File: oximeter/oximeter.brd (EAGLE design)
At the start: 29 x 41 mm, 24 parts, among them U1 AFE4490_AFE4490, U2 AZ1117EH-3.3TRG1, X1 FFC-32

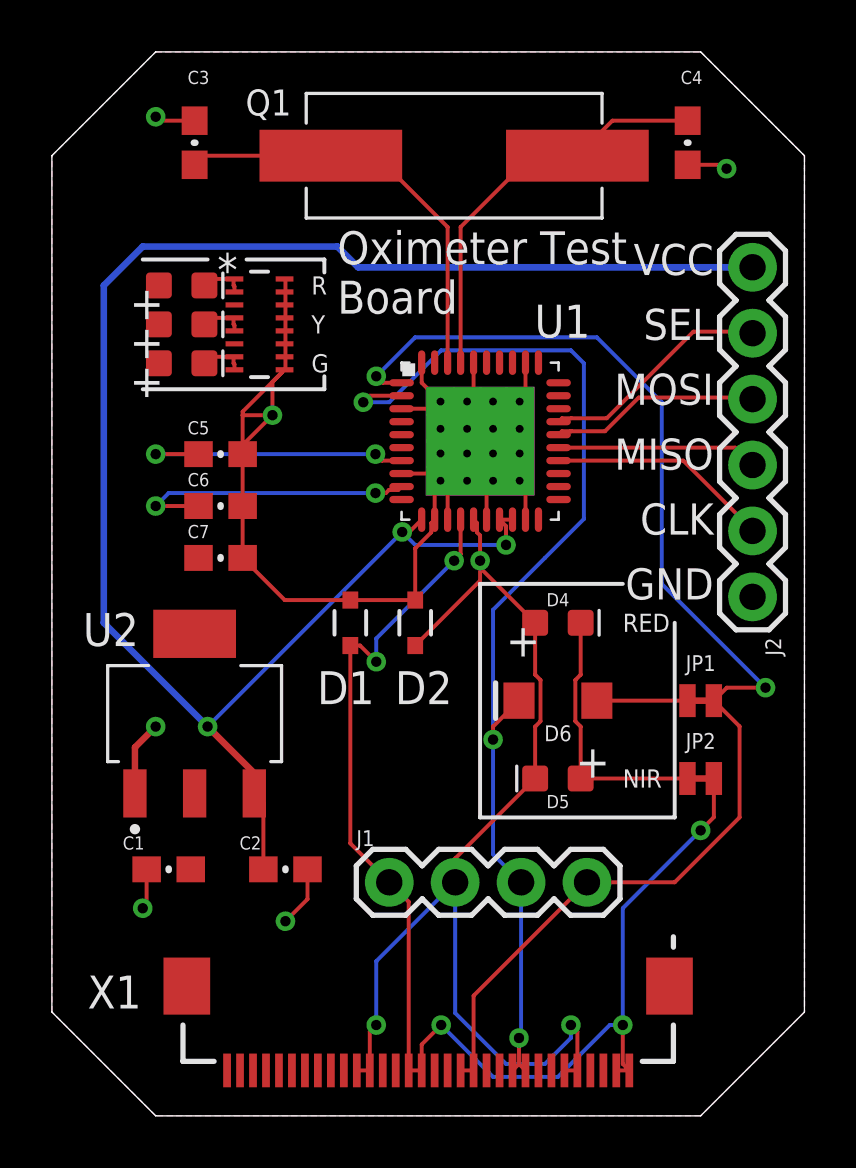
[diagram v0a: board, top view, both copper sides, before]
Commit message: more nextflex progress
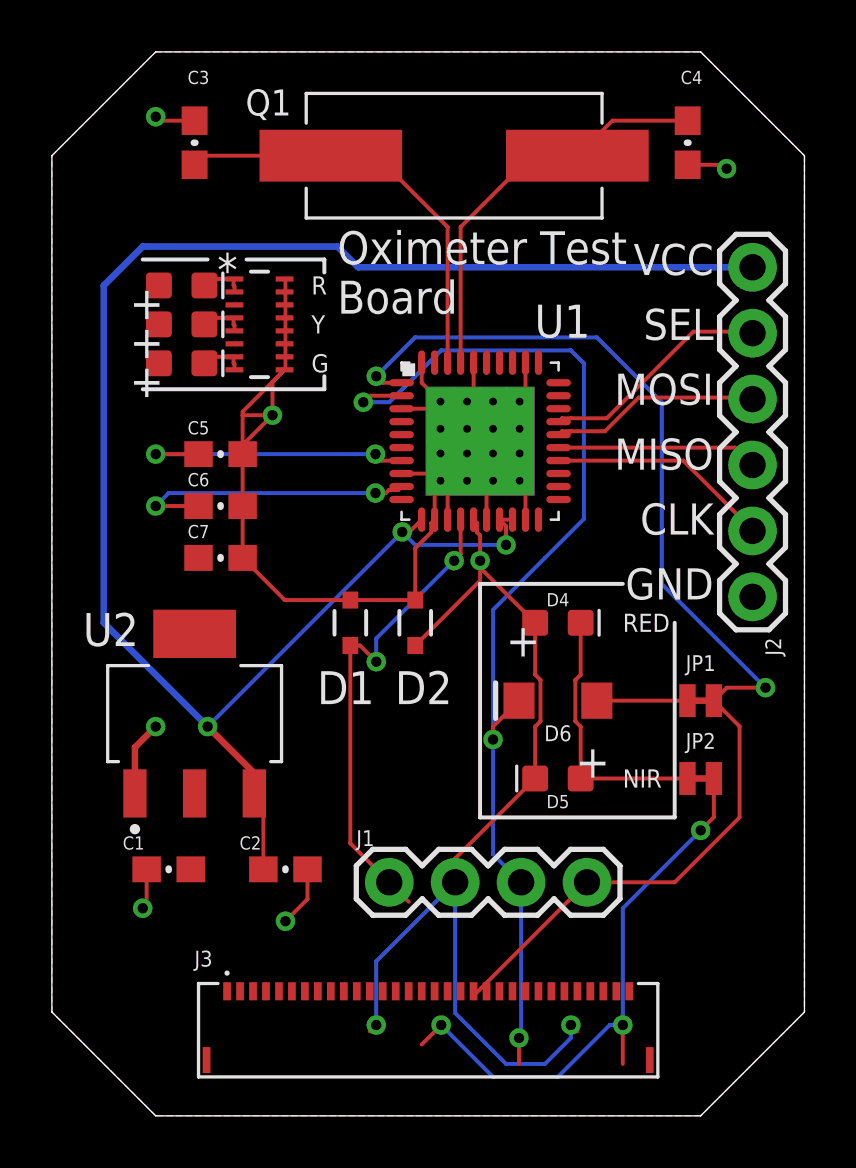
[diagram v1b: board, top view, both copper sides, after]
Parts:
- removed X1: FFC-32, scono:5034803200
- added J3: FFC-32, scono:MOLEX_503480-3200
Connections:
- new net N$1: J3.31
- new net N$2: J3.15
- new net N$3: J3.27
- new net N$4: J3.11
- new net N$8: J3.19
- new net N$9: J3.23
- net INN: now also J3.20; no longer X1.13, X1.14
- net INP: now also J3.24; no longer X1.10, X1.9
- net TXN: now also J3.16, J3.32; no longer X1.1, X1.17, X1.18, X1.2
- net TXP: now also J3.12, J3.28; no longer X1.21, X1.22, X1.5, X1.6
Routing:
- net TXN: track 49.9 -> 41.1 mm
- net TXP: track 43.4 -> 39.4 mm
- net INN: track 50.0 -> 46.6 mm
- net INP: track 42.7 -> 42.0 mm
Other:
- outline, holes or cut-outs redrawn
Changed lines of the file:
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@@
 <?xml version="1.0" encoding="utf-8"?>
 <!DOCTYPE eagle SYSTEM "eagle.dtd">
-<eagle version="9.4.2">
+<eagle version="9.5.1">
 <drawing>
 <settings>
@@
 <layer number="154" name="FabDoc2" color="7" fill="1" visible="yes" active="yes"/>
 <layer number="155" name="FabDoc3" color="7" fill="1" visible="yes" active="yes"/>
+<layer number="166" name="AntennaArea" color="7" fill="1" visible="no" active="yes"/>
+<layer number="168" name="4mmHeightArea" color="7" fill="1" visible="no" active="yes"/>
 <layer number="191" name="mNets" color="7" fill="1" visible="yes" active="yes"/>
 <layer number="192" name="mBusses" color="7" fill="1" visible="yes" active="yes"/>
@@
 <wire x1="3" y1="0" x2="24" y2="0" width="0" layer="20"/>
 <wire x1="24" y1="0" x2="28" y2="4" width="0" layer="20"/>
-<wire x1="28" y1="4" x2="28" y2="36.5" width="0" layer="20"/>
-<wire x1="28" y1="36.5" x2="28" y2="37" width="0" layer="20"/>
-<wire x1="28" y1="37" x2="27" y2="38" width="0" layer="20"/>
-<wire x1="27" y1="38" x2="24" y2="41" width="0" layer="20"/>
+<wire x1="28" y1="4" x2="28" y2="37" width="0" layer="20"/>
+<wire x1="28" y1="37" x2="24" y2="41" width="0" layer="20"/>
 <wire x1="24" y1="41" x2="3" y2="41" width="0" layer="20"/>
 <wire x1="3" y1="41" x2="-1" y2="37" width="0" layer="20"/>
@@
 <attribute name="VALUE" x="8.99356875" y="32.99531875" size="1.00116875" layer="27"/>
 </element>
-<element name="X1" library="scono" package="5034803200" value="FFC-32" x="13.5" y="5" smashed="yes" rot="R180">
-<attribute name="NAME" x="2.4476" y="5.405" size="1.27" layer="25" font="vector" rot="R180"/>
-<attribute name="VALUE" x="16.7476" y="5.8258" size="1.27" layer="27" font="vector" rot="R180"/>
-</element>
 <element name="U1" library="scono" package="AFE4490_QFN40-6X6" value="AFE4490_AFE4490" x="15.5" y="26" smashed="yes">
 <attribute name="NAME" x="17.6" y="29.99" size="1.27" layer="25" font="vector"/>
@@
 <attribute name="PROD_ID" value="CONN-09696" x="12" y="9" size="0.7" layer="27" font="vector" display="off"/>
 <attribute name="VALUE" x="10.73" y="6.968" size="0.6096" layer="27" font="vector" ratio="20"/>
+</element>
+<element name="J3" library="scono" library_urn="urn:adsk.eagle:library:14850048" package="MOLEX_503480-3200" package3d_urn="urn:adsk.eagle:package:14850860/1" value="FFC-32" x="13.5" y="3" smashed="yes">
+<attribute name="DESCRIPTION" value=" 0.50mm Pitch Easy-On™ BackFlip™ Type FPC Connector, 1.00mm Height, Right Angle, Surface Mount, Dual Contact Style, 32... " x="13.5" y="3" size="1.778" layer="27" display="off"/>
+<attribute name="DIGI-KEY_PART_NUMBER" value="WM11115CT-ND" x="13.5" y="3" size="1.778" layer="27" display="off"/>
+<attribute name="DIGI-KEY_PURCHASE_URL" value="https://www.digikey.com/product-detail/en/molex/5034803200/WM11115CT-ND/5171273?utm_source=snapeda&amp;utm_medium=aggregator&amp;utm_campaign=symbol" x="13.5" y="3" size="1.778" layer="27" display="off"/>
+<attribute name="MF" value="Molex" x="13.5" y="3" size="1.778" layer="27" display="off"/>
+<attribute name="MP" value="5034803200" x="13.5" y="3" size="1.778" layer="27" display="off"/>
+<attribute name="NAME" x="4.491259375" y="5.75266875" size="0.610190625" layer="25"/>
+<attribute name="PACKAGE" value="None" x="13.5" y="3" size="1.778" layer="27" display="off"/>
+<attribute name="VALUE" x="4.4939" y="0.498309375" size="0.6100125" layer="27"/>
 </element>
 </elements>
@@
 <contactref element="D1" pad="N"/>
 <contactref element="JP2" pad="2"/>
-<contactref element="X1" pad="1"/>
-<contactref element="X1" pad="2"/>
-<contactref element="X1" pad="17"/>
-<contactref element="X1" pad="18"/>
 <contactref element="J1" pad="1"/>
 <wire x1="14.75" y1="22.975" x2="14.75" y2="21.6432" width="0.1524" layer="1"/>
@@
 <via x="21" y="3.5" extent="1-16" drill="0.4"/>
 <wire x1="21" y1="3.5" x2="21" y2="2" width="0.1524" layer="1"/>
-<wire x1="21" y1="2" x2="21.25" y2="1.75" width="0.1524" layer="1"/>
-<wire x1="21.25" y1="1.75" x2="20.75" y2="1.75" width="0.1524" layer="1"/>
-<wire x1="12.75" y1="1.75" x2="13.25" y2="1.75" width="0.1524" layer="1"/>
 <wire x1="12" y1="9" x2="12.75" y2="8.25" width="0.1524" layer="1"/>
-<wire x1="12.75" y1="8.25" x2="12.75" y2="1.75" width="0.1524" layer="1"/>
 <wire x1="21" y1="3.5" x2="20.5" y2="3.5" width="0.1524" layer="16"/>
 <wire x1="20.5" y1="3.5" x2="18.5" y2="1.5" width="0.1524" layer="16"/>
@@
 <via x="14" y="3.5" extent="1-16" drill="0.4"/>
 <wire x1="14" y1="3.5" x2="13.25" y2="2.75" width="0.1524" layer="1"/>
-<wire x1="13.25" y1="2.75" x2="13.25" y2="1.75" width="0.1524" layer="1"/>
 <wire x1="12" y1="9" x2="10.5" y2="10.5" width="0.1524" layer="1"/>
 <wire x1="10.5" y1="10.5" x2="10.5" y2="18.1237" width="0.1524" layer="1"/>
@@
 <wire x1="11.5" y1="17.5" x2="10.8763" y2="18.1237" width="0.1524" layer="1"/>
 <wire x1="10.8763" y1="18.1237" x2="10.5" y2="18.1237" width="0.1524" layer="1"/>
+<contactref element="J3" pad="32"/>
+<contactref element="J3" pad="16"/>
+<wire x1="14" y1="3.5" x2="12.75" y2="8.25" width="0" layer="19" extent="1-1"/>
+<wire x1="21.25" y1="4.8" x2="13.25" y2="2.75" width="0" layer="19" extent="1-1"/>
+<wire x1="13.25" y1="4.8" x2="13.25" y2="2.75" width="0" layer="19" extent="1-1"/>
 </signal>
 <signal name="TXP">
@@
 <contactref element="D5" pad="C"/>
 <contactref element="D4" pad="A"/>
-<contactref element="X1" pad="5"/>
-<contactref element="X1" pad="6"/>
-<contactref element="X1" pad="21"/>
-<contactref element="X1" pad="22"/>
 <contactref element="J1" pad="2"/>
 <via x="15.5" y="21.3932" extent="1-16" drill="0.4"/>
@@
 <wire x1="17.623" y1="19" x2="15.5" y2="21.123" width="0.1524" layer="1"/>
 <wire x1="15.5" y1="21.123" x2="15.5" y2="21.3932" width="0.1524" layer="1"/>
-<wire x1="10.75" y1="1.75" x2="11.25" y2="1.75" width="0.1524" layer="1"/>
-<wire x1="19.25" y1="1.75" x2="19.25" y2="3.25" width="0.1524" layer="1"/>
 <wire x1="19.25" y1="3.25" x2="19" y2="3.5" width="0.1524" layer="1"/>
 <via x="19" y="3.5" extent="1-16" drill="0.4"/>
-<wire x1="19.25" y1="1.75" x2="18.75" y2="1.75" width="0.1524" layer="1"/>
-<wire x1="11.25" y1="1.75" x2="11.25" y2="3.25" width="0.1524" layer="1"/>
 <wire x1="11.25" y1="3.25" x2="11.5" y2="3.5" width="0.1524" layer="1"/>
 <via x="11.5" y="3.5" extent="1-16" drill="0.4"/>
@@
 <wire x1="13" y1="18.1237" x2="15.5" y2="20.6237" width="0.1524" layer="1"/>
 <wire x1="15.5" y1="20.6237" x2="15.5" y2="21.3932" width="0.1524" layer="1"/>
+<contactref element="J3" pad="28"/>
+<contactref element="J3" pad="12"/>
+<wire x1="19.25" y1="4.8" x2="11.25" y2="3.25" width="0" layer="19" extent="1-1"/>
+<wire x1="11.25" y1="4.8" x2="11.25" y2="3.25" width="0" layer="19" extent="1-1"/>
 </signal>
 <signal name="XIN">
@@
 <contactref element="U1" pad="1"/>
 <contactref element="JP1" pad="2"/>
-<contactref element="X1" pad="13"/>
-<contactref element="X1" pad="14"/>
 <contactref element="J1" pad="4"/>
 <wire x1="12.475" y1="28.25" x2="11.75" y2="28.25" width="0.1524" layer="1"/>
@@
 <wire x1="23" y1="9" x2="19.62" y2="9" width="0.1524" layer="1"/>
 <wire x1="19.62" y1="9" x2="15.25" y2="4.63" width="0.1524" layer="1"/>
-<wire x1="15.25" y1="4.63" x2="15.25" y2="1.75" width="0.1524" layer="1"/>
 <wire x1="24.508" y1="16" x2="25.008" y2="16.5" width="0.1524" layer="1"/>
 <wire x1="25.008" y1="16.5" x2="26.5" y2="16.5" width="0.1524" layer="1"/>
@@
 <wire x1="11.5" y1="28.5" x2="13" y2="30" width="0.1524" layer="16"/>
 <wire x1="13" y1="30" x2="20" y2="30" width="0.1524" layer="16"/>
-<wire x1="14.75" y1="1.75" x2="15.25" y2="1.75" width="0.1524" layer="1"/>
+<contactref element="J3" pad="20"/>
+<wire x1="15.25" y1="4.8" x2="15.25" y2="4.63" width="0" layer="19" extent="1-1"/>
 </signal>
 <signal name="BG">
@@
 <contactref element="U1" pad="2"/>
 <contactref element="D6" pad="C"/>
-<contactref element="X1" pad="9"/>
-<contactref element="X1" pad="10"/>
 <contactref element="J1" pad="3"/>
 <wire x1="12.475" y1="27.75" x2="11.25" y2="27.75" width="0.1524" layer="1"/>
@@
 <via x="17" y="3" extent="1-16" drill="0.4"/>
 <wire x1="17" y1="3" x2="17" y2="2" width="0.1524" layer="1"/>
-<wire x1="17" y1="2" x2="16.75" y2="1.75" width="0.1524" layer="1"/>
-<wire x1="17.25" y1="1.75" x2="17" y2="2" width="0.1524" layer="1"/>
 <wire x1="17.08" y1="9" x2="16" y2="10.08" width="0.1524" layer="16"/>
 <wire x1="16" y1="10.08" x2="16" y2="14.5" width="0.1524" layer="16"/>
@@
 <wire x1="14" y1="29.5" x2="12" y2="27.5" width="0.1524" layer="16"/>
 <wire x1="12" y1="27.5" x2="11" y2="27.5" width="0.1524" layer="16"/>
+<contactref element="J3" pad="24"/>
+<wire x1="17.25" y1="4.8" x2="17" y2="2" width="0" layer="19" extent="1-1"/>
 </signal>
 <signal name="ADC_RDY">
@@
 <wire x1="23.492" y1="13" x2="19.377" y2="13" width="0.1524" layer="1"/>
 </signal>
+<signal name="N$1">
+<contactref element="J3" pad="31"/>
+</signal>
+<signal name="N$2">
+<contactref element="J3" pad="15"/>
+</signal>
+<signal name="N$3">
+<contactref element="J3" pad="27"/>
+</signal>
+<signal name="N$4">
+<contactref element="J3" pad="11"/>
+</signal>
+<signal name="N$8">
+<contactref element="J3" pad="19"/>
+</signal>
+<signal name="N$9">
+<contactref element="J3" pad="23"/>
+</signal>
 </signals>
 <mfgpreviewcolors>
@@
 which will not be processed correctly with this version.
 </note>
+<note version="8.2" severity="warning">
+Since Version 8.2, EAGLE supports online libraries. The ids
+of those online libraries will not be understood (or retained)
+with this version.
+</note>
 <note version="8.3" severity="warning">
